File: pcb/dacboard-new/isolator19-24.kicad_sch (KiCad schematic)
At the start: 18 parts, among them U100 ISO6761FQDWRQ1, U101 ISO6761FQDWRQ1, U102 ISO6761FQDWRQ1, U103 ISO6761FQDWRQ1, U104 ISO6761FQDWRQ1, U105 ISO6761FQDWRQ1

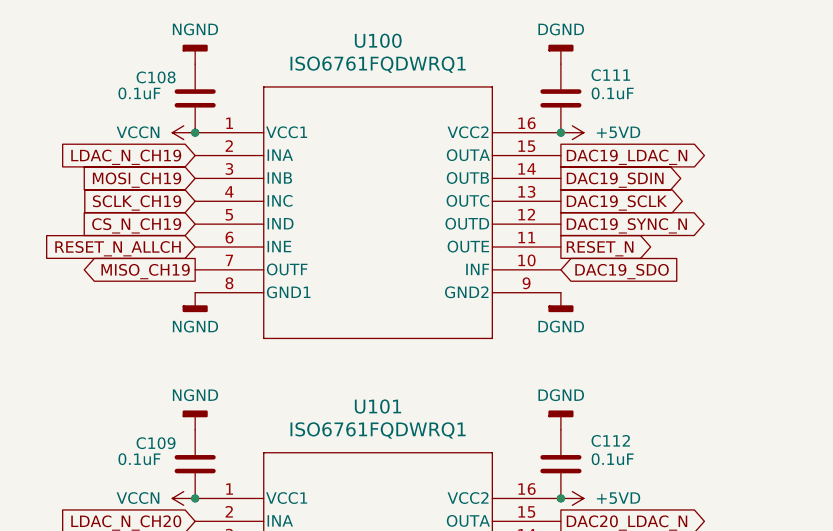
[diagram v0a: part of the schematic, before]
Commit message: cleared drc
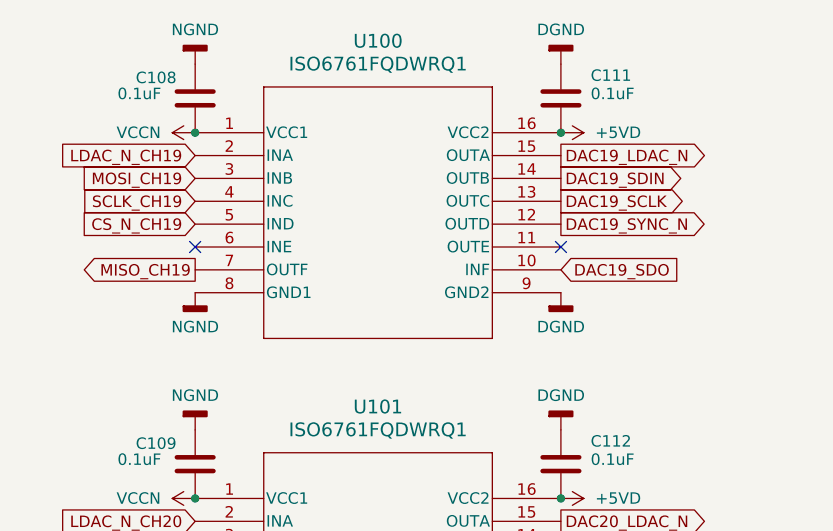
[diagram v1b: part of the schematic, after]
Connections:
- net RESET_N: no longer names the net of U100.11 (OUTE)
- net RESET_N_ALLCH: no longer names the net of U100.6 (INE)
- no-connect marks 10 -> 12
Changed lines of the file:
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@@
+	)
+	(no_connect
+		(at 74.93 57.15)
 	)
 	(no_connect
@@
 	)
 	(no_connect
+		(at 115.57 57.15)
+	)
+	(no_connect
 		(at 74.93 97.79)
 	)
@@
 			(effects
 				(font
-					(size 1.27 1.27)
-				)
-				(justify right)
-				(hide yes)
-			)
-		)
-	)
-	(global_label "RESET_N"
-		(shape output)
-		(at 115.57 57.15 0)
-		(fields_autoplaced yes)
-		(effects
-			(font
-				(size 1.27 1.27)
-			)
-			(justify left)
-		)
-		(property "Intersheetrefs" "${INTERSHEET_REFS}"
-			(at 126.5984 57.15 0)
-			(effects
-				(font
-					(size 1.27 1.27)
-				)
-				(justify left)
-				(hide yes)
-			)
-		)
-	)
-	(global_label "RESET_N_ALLCH"
-		(shape input)
-		(at 74.93 57.15 180)
-		(fields_autoplaced yes)
-		(effects
-			(font
-				(size 1.27 1.27)
-			)
-			(justify right)
-		)
-		(property "Intersheetrefs" "${INTERSHEET_REFS}"
-			(at 57.1887 57.15 0)
-			(effects
-				(font
